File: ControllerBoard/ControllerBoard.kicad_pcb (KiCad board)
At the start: 4 copper layers, 34 x 12 mm, 31 parts, among them J1 X0511WVS-24AS-LPV01, J2 X0511WVS-24AS-LPV01, U1 PLP5860RKPR, U2 LIS2DE12, U3 nRF52810-QCxx, Y1 32.768kHz 12.5pF, Y2 32MHz 8pF <40ppm

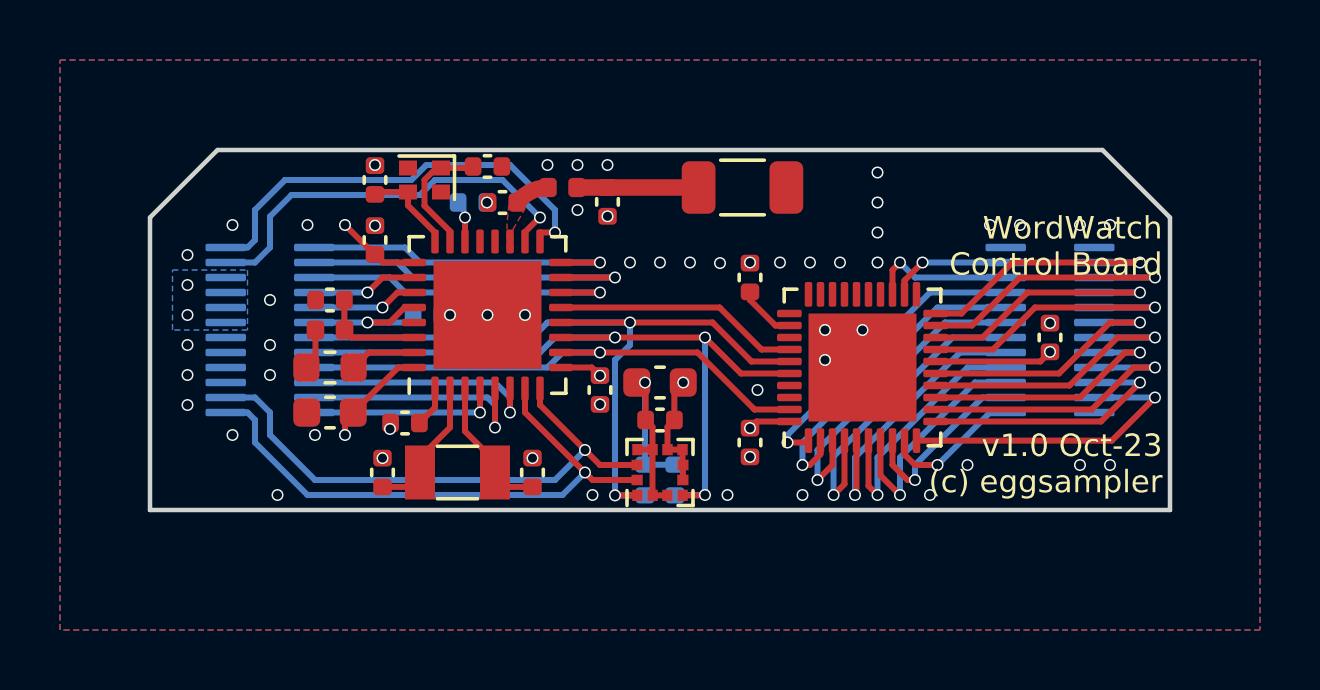
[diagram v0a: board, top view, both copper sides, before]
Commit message: Minor board updates
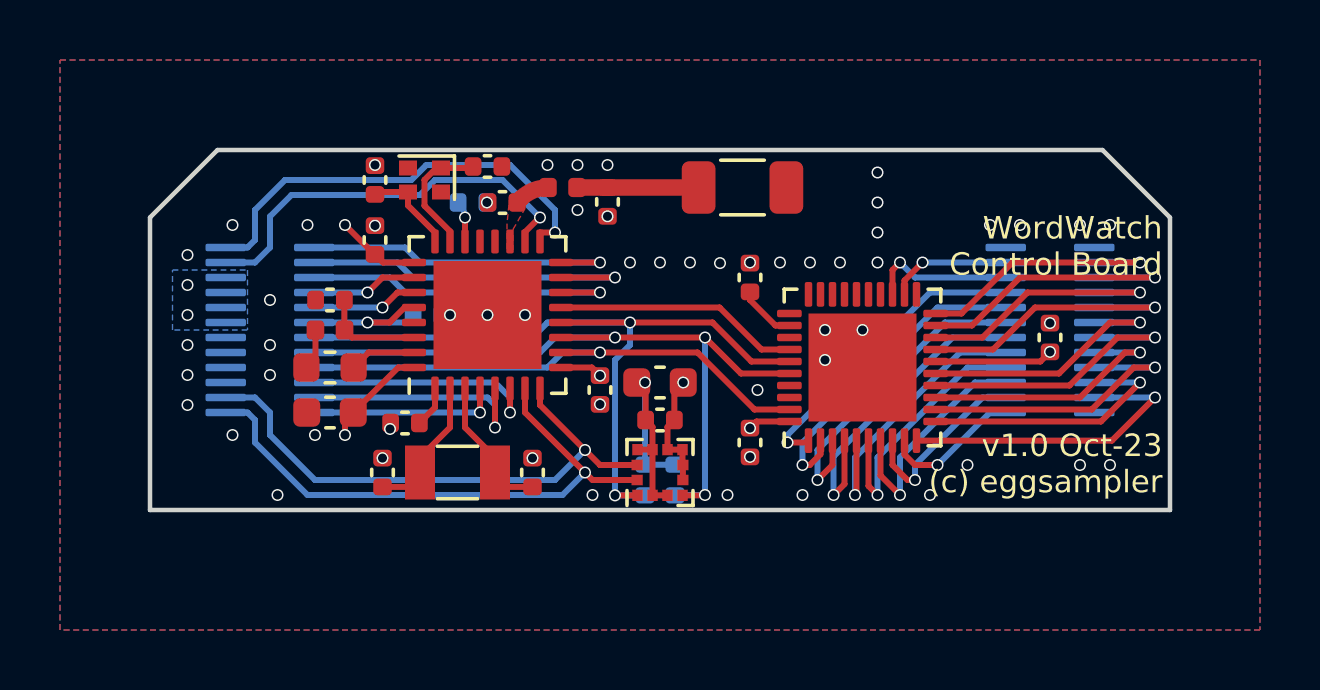
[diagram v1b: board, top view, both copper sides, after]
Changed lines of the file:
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@@
   (segment (start 135.27 76.75) (end 135.309081 76.789081) (width 0.2) (layer "B.Cu") (net 6))
   (arc (start 135.309081 76.789081) (mid 135.450381 77.000552) (end 135.5 77.25) (width 0.2) (layer "B.Cu") (net 6))
+  (segment (start 134 85.25) (end 134 85.75) (width 0.2) (layer "F.Cu") (net 7))
+  (segment (start 135 82.95) (end 135 84.25) (width 0.2) (layer "F.Cu") (net 7))
   (segment (start 134 86.23) (end 134 85.75) (width 0.2) (layer "F.Cu") (net 7))
   (segment (start 132.75 86.23) (end 134 86.23) (width 0.2) (layer "F.Cu") (net 7))
   (segment (start 135 84.25) (end 134 85.25) (width 0.2) (layer "F.Cu") (net 7))
-  (segment (start 135 82.95) (end 135 84.25) (width 0.2) (layer "F.Cu") (net 7))
-  (segment (start 134 85.25) (end 134 85.75) (width 0.2) (layer "F.Cu") (net 7))
   (segment (start 136.5 86.23) (end 136.5 85.75) (width 0.2) (layer "F.Cu") (net 8))
-  (segment (start 135.5 84.375) (end 136.5 85.375) (width 0.2) (layer "F.Cu") (net 8))
-  (segment (start 135.5 82.95) (end 135.5 84.375) (width 0.2) (layer "F.Cu") (net 8))
+  (segment (start 135.5 82.95) (end 135.5 84.25) (width 0.2) (layer "F.Cu") (net 8))
+  (segment (start 135.5 84.25) (end 136.5 85.25) (width 0.2) (layer "F.Cu") (net 8))
+  (segment (start 136.5 85.25) (end 136.5 85.75) (width 0.2) (layer "F.Cu") (net 8))
   (segment (start 137.75 86.23) (end 136.5 86.23) (width 0.2) (layer "F.Cu") (net 8))
-  (segment (start 136.5 85.375) (end 136.5 85.75) (width 0.2) (layer "F.Cu") (net 8))
   (segment (start 134.5 83.58) (end 133.98 84.1) (width 0.2) (layer "F.Cu") (net 9))
   (segment (start 134.5 82.95) (end 134.5 83.58) (width 0.2) (layer "F.Cu") (net 9))
